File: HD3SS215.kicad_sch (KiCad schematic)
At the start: 23 parts, among them U1 HD3SS215

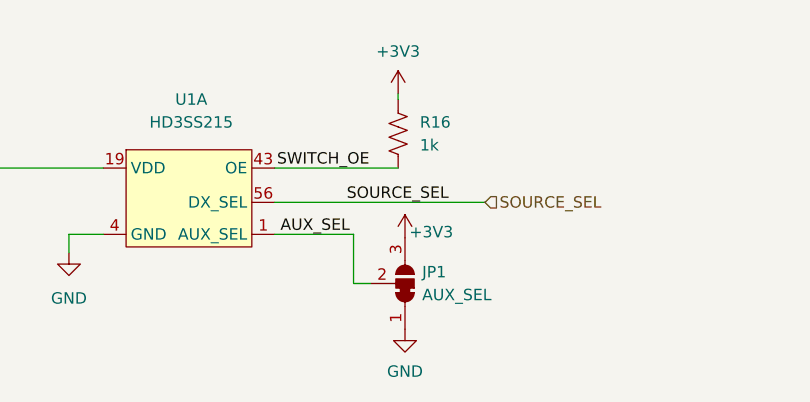
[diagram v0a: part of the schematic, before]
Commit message: Pushing what i have now
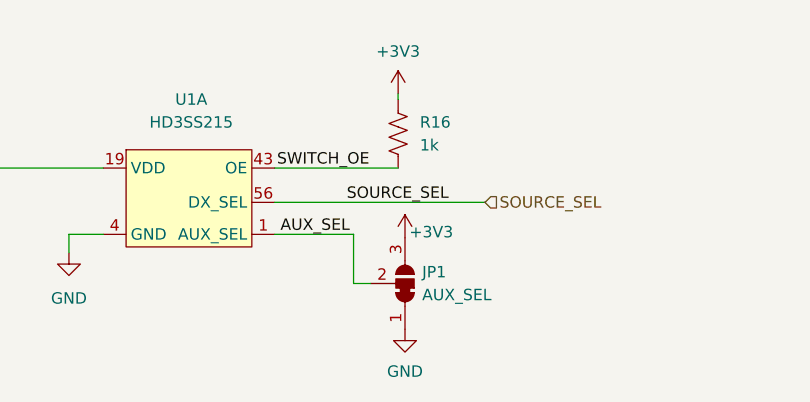
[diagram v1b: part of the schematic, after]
